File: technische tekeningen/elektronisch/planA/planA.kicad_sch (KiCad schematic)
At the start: 20 parts, among them J1 Connector_usb-serial, M1 Motor_DC, M2 Motor_DC, SW1 reset, U1 ESP32-S3-WROOM-1, U2 AMS1117-3.3

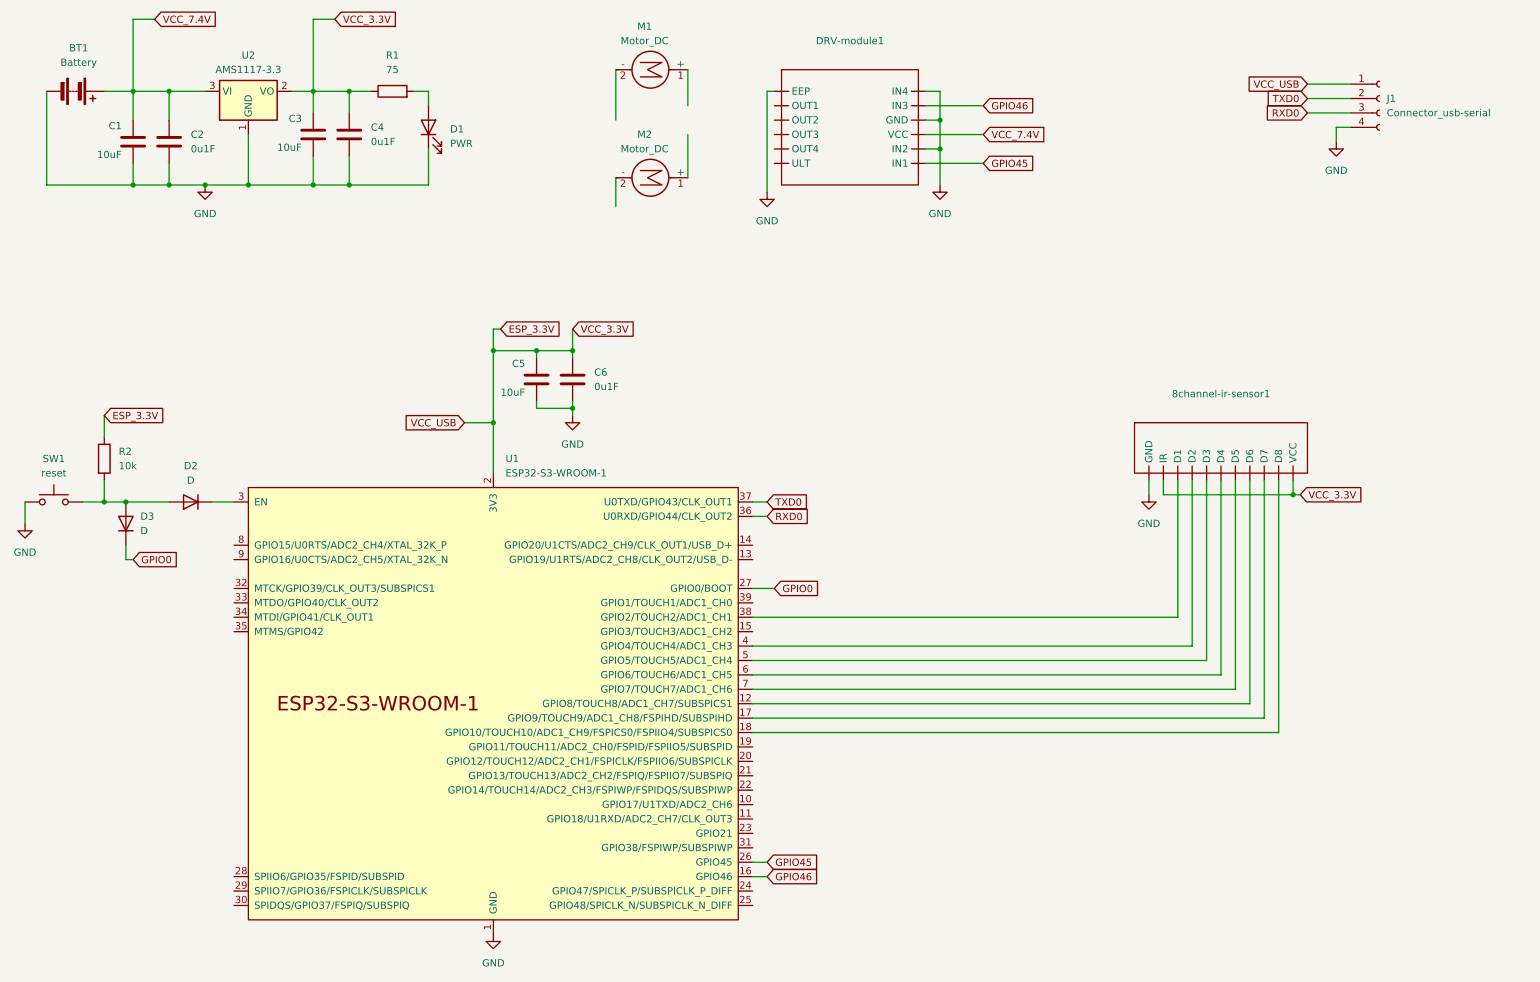
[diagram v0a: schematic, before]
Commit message: update
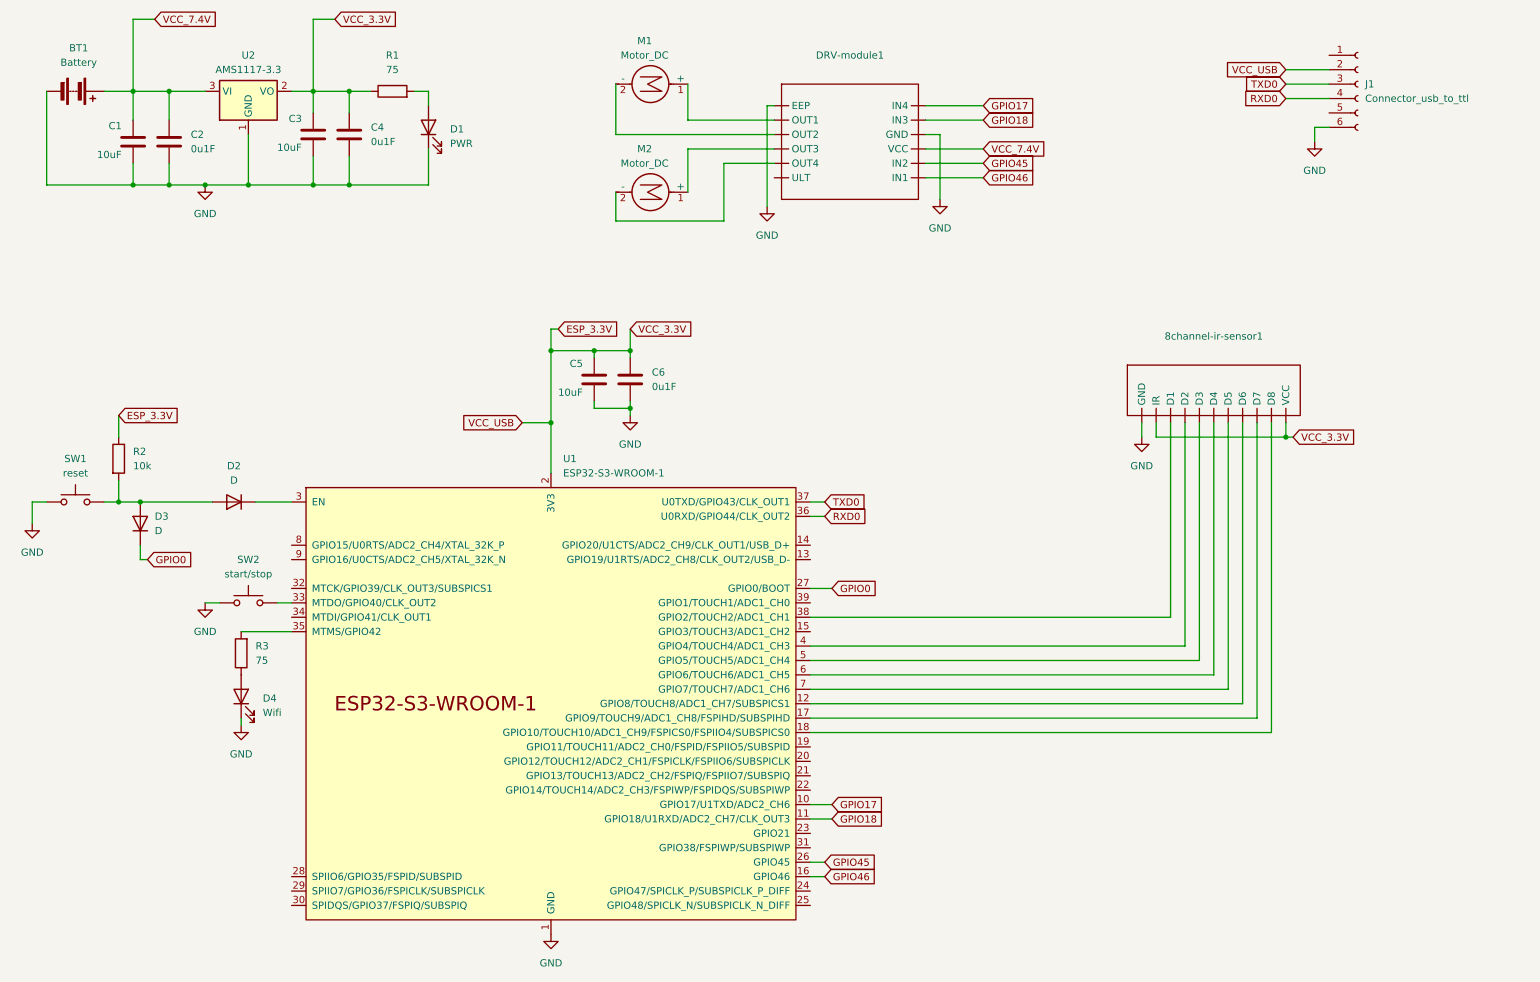
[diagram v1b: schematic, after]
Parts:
- removed J1: Connector_usb-serial, symbol Connector:Conn_01x04_Socket
- added D4: Wifi, LED_THT:LED_D5.0mm, symbol Device:LED
- added J1: Connector_usb_to_ttl, symbol Connector:Conn_01x06_Socket
- added R3: 75, Resistor_THT:R_Axial_DIN0204_L3.6mm_D1.6mm_P7.62mm_Horizontal, symbol Device:R
- added SW2: start/stop, Button_Switch_SMD:SW_SPST_PTS645Sx43SMTR92, symbol Switch:SW_Push
- D1: footprint (none) -> LED_THT:LED_D5.0mm
- R1, R2: footprint (none) -> Resistor_THT:R_Axial_DIN0204_L3.6mm_D1.6mm_P7.62mm_Horizontal
- SW1: footprint (none) -> Button_Switch_SMD:SW_SPST_PTS645Sx43SMTR92
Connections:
- net ESP_3.3V: now also J1.2 (Pin_2)
- net GND: now also D4.1 (K), J1.6 (Pin_6), SW2.1
- net RXD0: now also J1.4 (Pin_4)
- net TXD0: now also J1.3 (Pin_3)
- net at M2.1 (+): now also DRV-module1. (IN1)
- net at M2.2 (-): now also DRV-module1. (IN1)
- net at M1.1 (+): now also DRV-module1. (IN1)
- net at M1.2 (-): now also DRV-module1. (IN1)
- net GPIO17: now reaches U1.10 (GPIO17/U1TXD/ADC2_CH6)
- net GPIO17: now also DRV-module1. (IN1)
- net GPIO18: now reaches U1.11 (GPIO18/U1RXD/ADC2_CH7/CLK_OUT3)
- net GPIO18: now also DRV-module1. (IN1)
- net at U1.33 (MTDO/GPIO40/CLK_OUT2): now also SW2.2
- net at U1.35 (MTMS/GPIO42): now also R3.2
- new net: D4.2 (A), R3.1
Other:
- moved on the sheet: 8channel-ir-sensor1, C5, C6, D2, D3, DRV-module1, M1, M2, R2, SW1, U1
